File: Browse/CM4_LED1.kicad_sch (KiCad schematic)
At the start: 3 parts, among them U3 Buffers & Line Driver

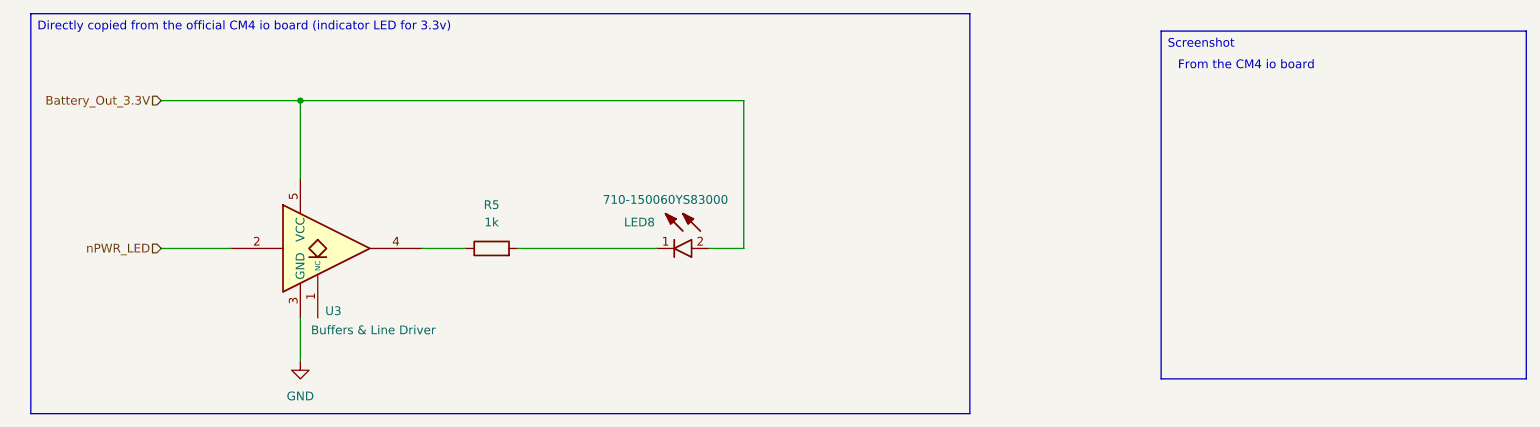
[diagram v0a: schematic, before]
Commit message: Deploying to gh-pages from @ Nautilus-UUV/nautilus-mainboard-PCB@5f5fdd9436d408a604bb268d740c0ac7ce1f5af5 🚀
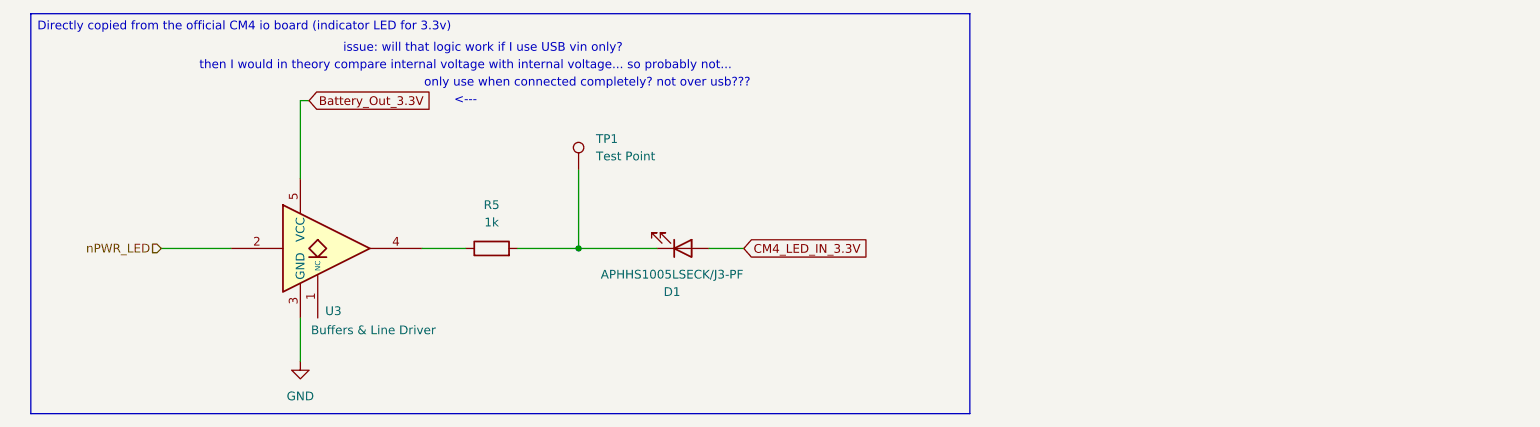
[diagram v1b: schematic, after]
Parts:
- removed LED8: 710-150060YS83000, dz_dio:Wuerth_LED_150060RS83000, symbol #dzdb:s_dio/D-WURT-710-150060YS83000
- added D1: APHHS1005LSECK/J3-PF, LED_SMD:LED_0402_1005Metric, symbol #dzdb:s_dio/D-KIN-APHHS1005LSECK/J3-PF
- added TP1: Test Point, TestPoint:TestPoint_Pad_D1.5mm, symbol #dzdb:g_mech/M-TEST-SMT_1.5mm_round
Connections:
- net at R5.2: now also D1.1 (K), TP1.1
- new net CM4_LED_IN_3.3V: D1.2 (A)
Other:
- note added: "<---"
- note added: "issue: will that logic work if I use USB vin only?"
- note added: "only use when connected completely? not over usb???"
- note added: "then I would in theory compare internal voltage with internal voltage... so probably not..."
- note removed: "From the CM4 io board"
- company: Davide -> (none)
- title: Nautilus_Mainboard -> (none)

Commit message: Deploying to gh-pages from @ Nautilus-UUV/nautilus-mainboard-PCB@f1dd6ce1e57c066b805694b10777c719502cca87 🚀
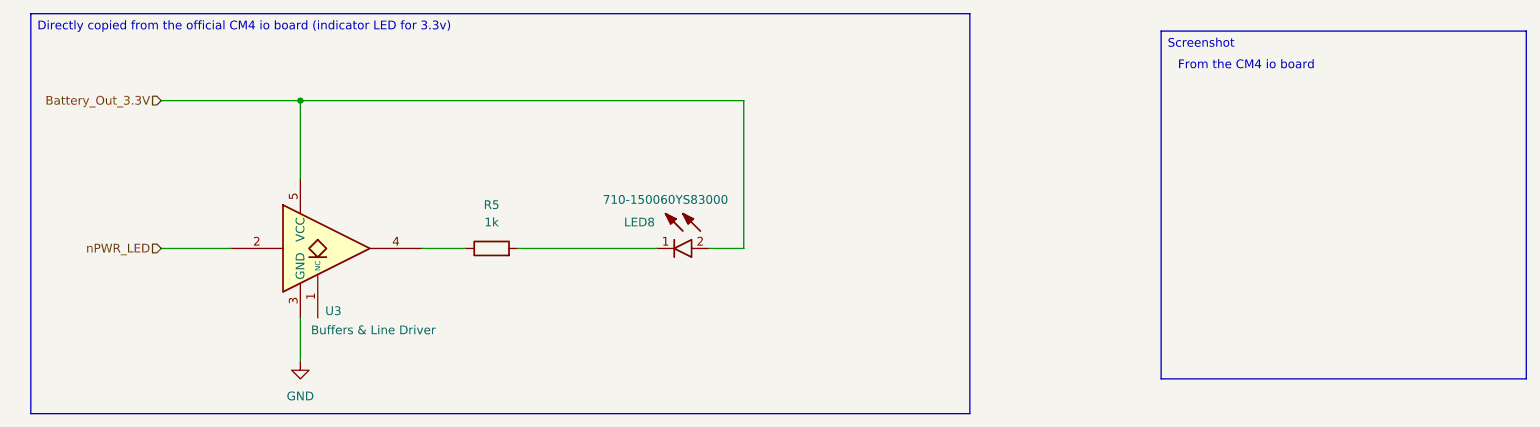
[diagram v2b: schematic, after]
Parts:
- removed D1: APHHS1005LSECK/J3-PF, LED_SMD:LED_0402_1005Metric, symbol #dzdb:s_dio/D-KIN-APHHS1005LSECK/J3-PF
- removed TP1: Test Point, TestPoint:TestPoint_Pad_D1.5mm, symbol #dzdb:g_mech/M-TEST-SMT_1.5mm_round
- added LED8: 710-150060YS83000, dz_dio:Wuerth_LED_150060RS83000, symbol #dzdb:s_dio/D-WURT-710-150060YS83000
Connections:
- net Battery_Out_3.3V: now also LED8.2 (A)
- net at R5.2: now also LED8.1 (K)
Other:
- note added: "From the CM4 io board"
- note removed: "<---"
- note removed: "issue: will that logic work if I use USB vin only?"
- note removed: "only use when connected completely? not over usb???"
- note removed: "then I would in theory compare internal voltage with internal voltage... so probably not..."
- company: (none) -> Davide
- title: (none) -> Nautilus_Mainboard
